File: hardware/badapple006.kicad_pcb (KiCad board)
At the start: 2 copper layers, 16.5 x 16.2 mm, 35 parts, among them J10 5V, J11 GND, J12 RB066-6448-TSWHG01, J2 USB_C_Receptacle_USB2.0, J3 PG, J4 3v3, J5 GND, J6 RFO, J7 RFA, J8 APPLE, J9 RFO2, U1 CH32V006F8U7, U2 XC6206P362, Y1 24MHz

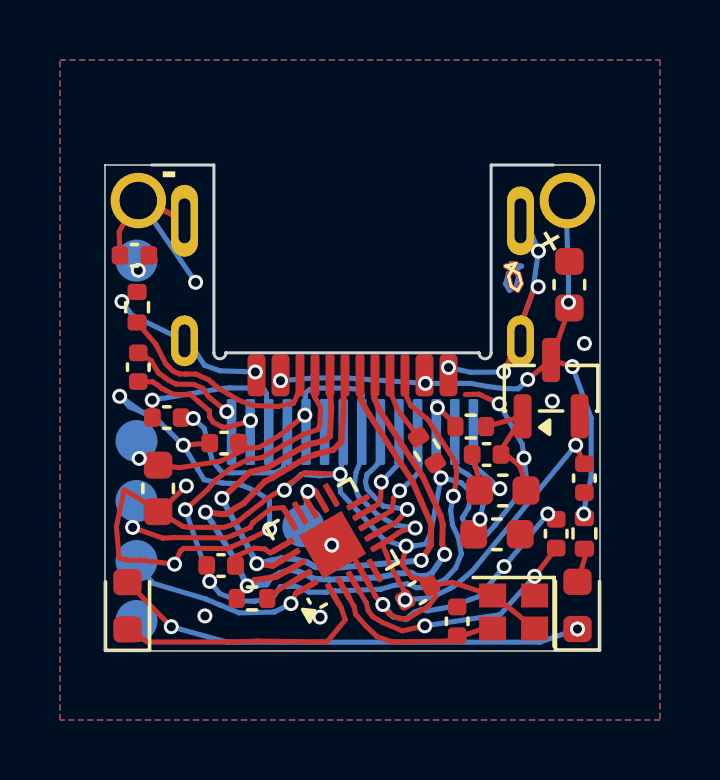
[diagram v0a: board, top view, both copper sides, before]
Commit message: Update hardware
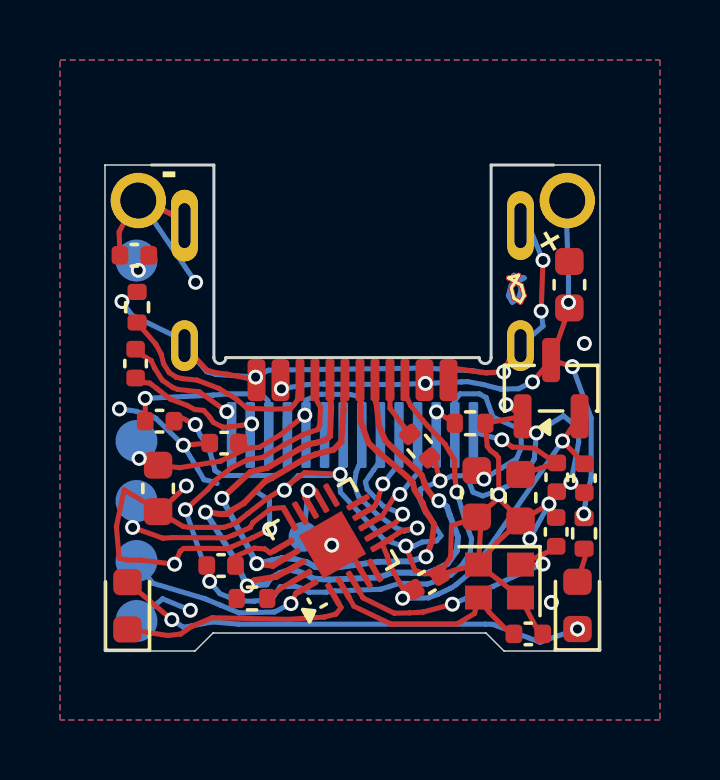
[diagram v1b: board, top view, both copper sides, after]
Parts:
- moved C18 2.46 mm to (85.1, 90.4), turned to -90 degrees
- moved C10 2.41 mm to (84.1, 95.6), turned to 180 degrees
- moved C11 1.51 mm to (82.4, 91.0), turned to -90 degrees
- moved Y1 1.13 mm to (83.2, 93.9)
- moved C17 0.64 mm to (83.8, 91.1), turned to -90 degrees
- moved C16 0.47 mm to (80.7, 93.9)
- moved J9 0.35 mm to (76.6, 92.4)
- moved R2 0.27 mm to (80.5, 89.4), turned to -50 degrees
- moved C14 0.27 mm to (71.8, 88.5)
- moved J2 0.16 mm to (78.2, 81.8)
- moved C13 0.15 mm to (71.0, 86.6)
- moved R1 0.11 mm to (82.2, 88.6)
- moved J12 0.10 mm to (78.2, 89.0)
- moved C9 0.06 mm to (85.0, 92.2)
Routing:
- net GND: track 93.0 -> 105.3 mm, vias 26 -> 25
- net Net-(J12-Pin_13): track 5.01 -> 7.61 mm
- net Net-(U1-PA1/T1/T2/OPN0/XI/A1): track 5.65 -> 7.12 mm
- net REDCOLOR: track 8.67 -> 7.90 mm
- net D-: track 27.0 -> 27.6 mm
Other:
- outline, holes or cut-outs redrawn
- board text added: "* Red 1.2mm thick * OSP or ENIG * 5x5 with side rails"
- board text added: "rev bad"
- board text removed: "rev b"
